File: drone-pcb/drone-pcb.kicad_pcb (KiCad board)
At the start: 2 copper layers, 100 x 100 mm, 26 parts, among them J1 MOT_1, J2 MOT_2, J3 MOT_3, J4 MOT_4, J5 BAT, Q1 AO3400A, Q2 AO3400A, Q3 AO3400A, Q4 AO3400A, U1 XIAO ESP32C3

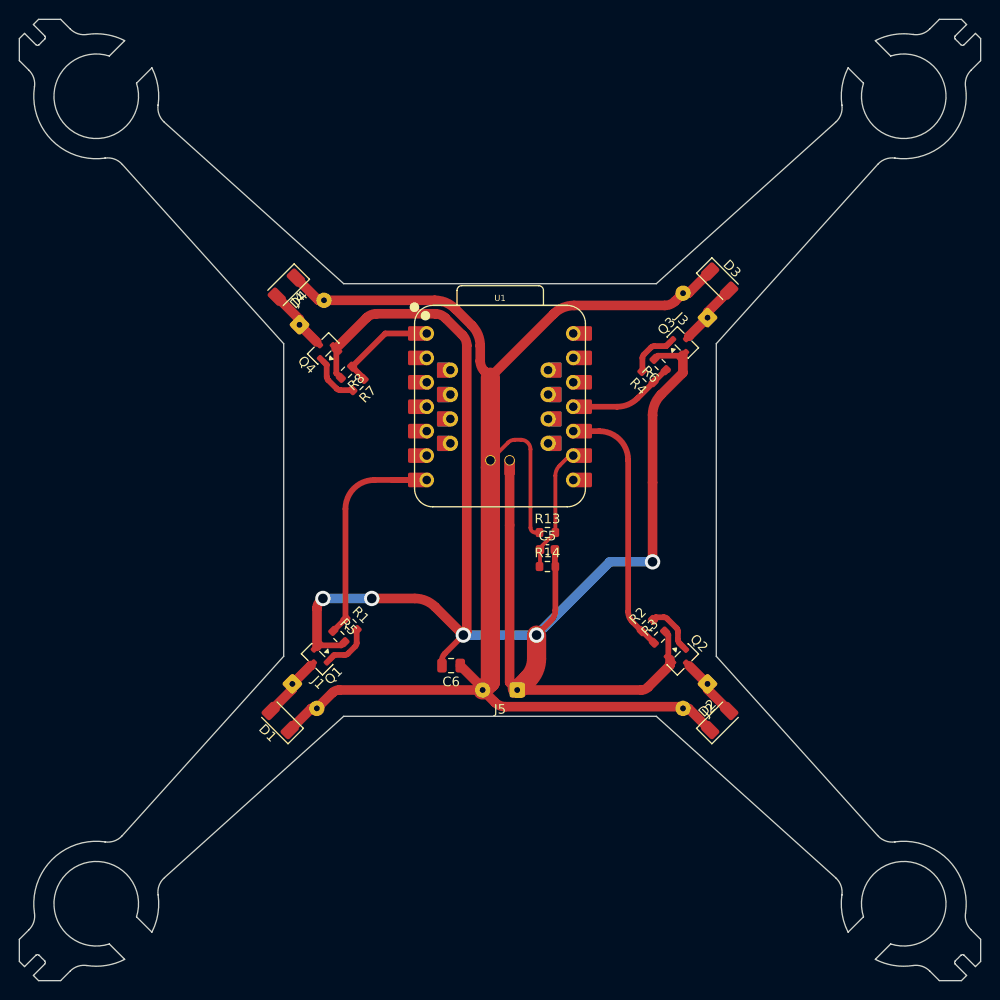
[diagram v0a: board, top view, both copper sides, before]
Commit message: uptodate_pcb_v1.0
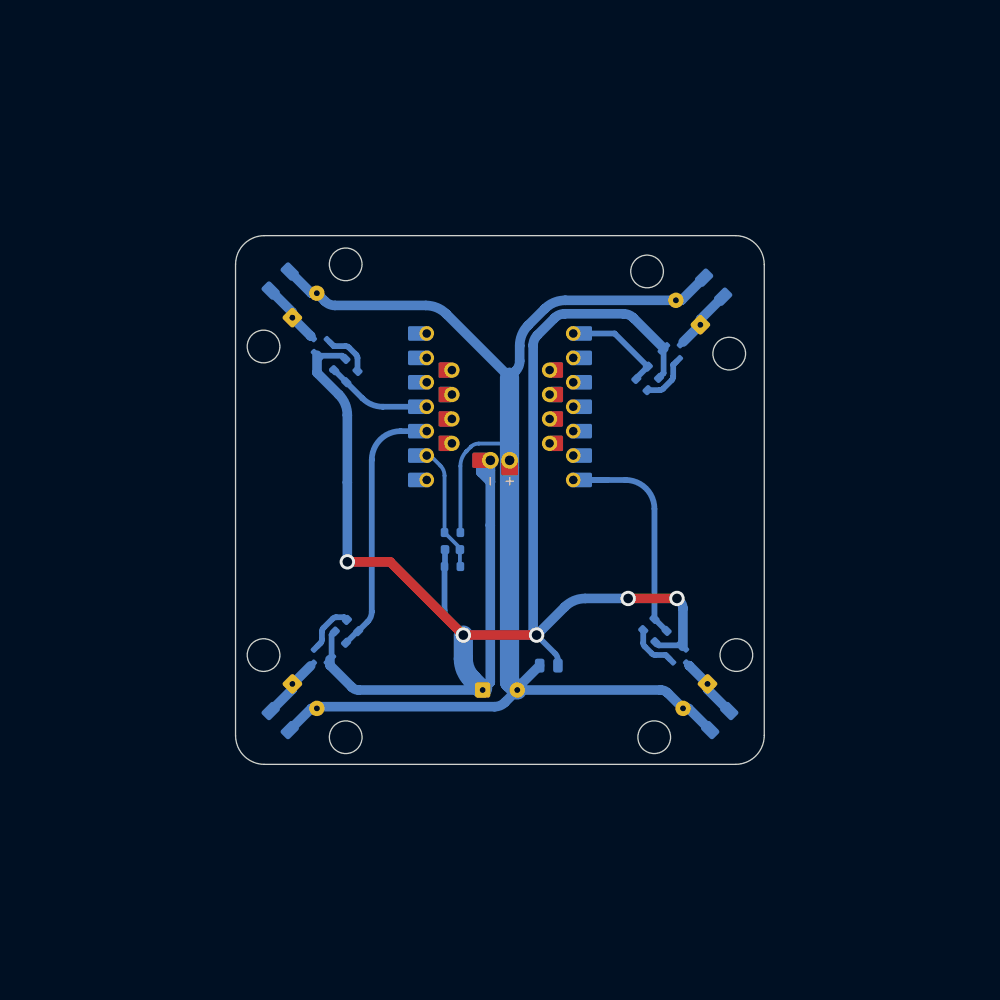
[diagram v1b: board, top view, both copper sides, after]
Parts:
- C5, C6, D1, D2, D3, D4, J1, J2, J3, J4, J5, Q1, Q2, Q3, Q4, R1, R13, R14, R2, R3, R4, R5, R6, R7, R8, U1: moved to B.Cu
- moved D1 45.7 mm to (139.0, 94.9), turned to 45 degrees
- moved D2 45.7 mm to (93.2, 94.9), turned to 135 degrees
- moved D3 45.7 mm to (93.2, 49.1), turned to -135 degrees
- moved D4 44.4 mm to (138.3, 49.8), turned to -45 degrees
- moved J1 43.2 mm to (137.7, 91.0), turned to -135 degrees
- moved J3 43.2 mm to (94.5, 52.9), turned to 45 degrees
- moved J2 43.2 mm to (94.5, 91.0), turned to -45 degrees
- moved J4 41.7 mm to (137.0, 53.7), turned to 135 degrees
- moved Q1 38.0 mm to (135.1, 88.5), turned to -45 degrees
- moved Q2 38.0 mm to (97.1, 88.5), turned to -135 degrees
- moved Q3 38.0 mm to (97.1, 55.5), turned to 135 degrees
- moved Q4 36.8 mm to (134.5, 56.2), turned to 45 degrees
- moved R5 33.5 mm to (132.9, 86.1), turned to -135 degrees
- moved R6 33.3 mm to (99.5, 57.8), turned to 45 degrees
- moved R3 33.2 mm to (99.5, 86.2), turned to 135 degrees
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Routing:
- net GND: track 187.0 -> 193.4 mm
- net V_BAT: track 152.2 -> 150.7 mm
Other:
- board size 100 x 100 mm -> 55 x 55 mm
